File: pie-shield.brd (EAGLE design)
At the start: 35.1 x 25.2 mm, 21 parts, among them IC1 MAX481CSA, IC4 NRF24L01SMD, Q2 3.2X2.5CRYSTAL

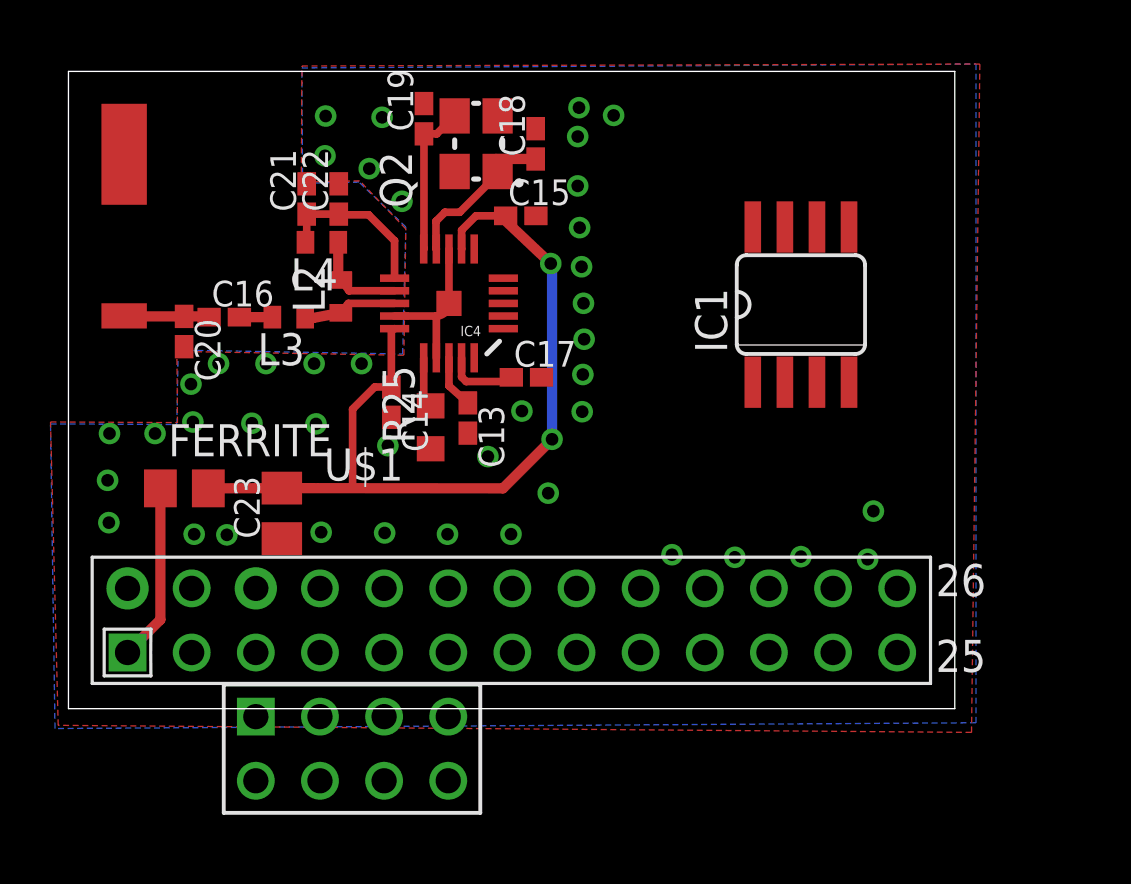
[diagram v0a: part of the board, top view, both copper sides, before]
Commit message: 1 square inch reached
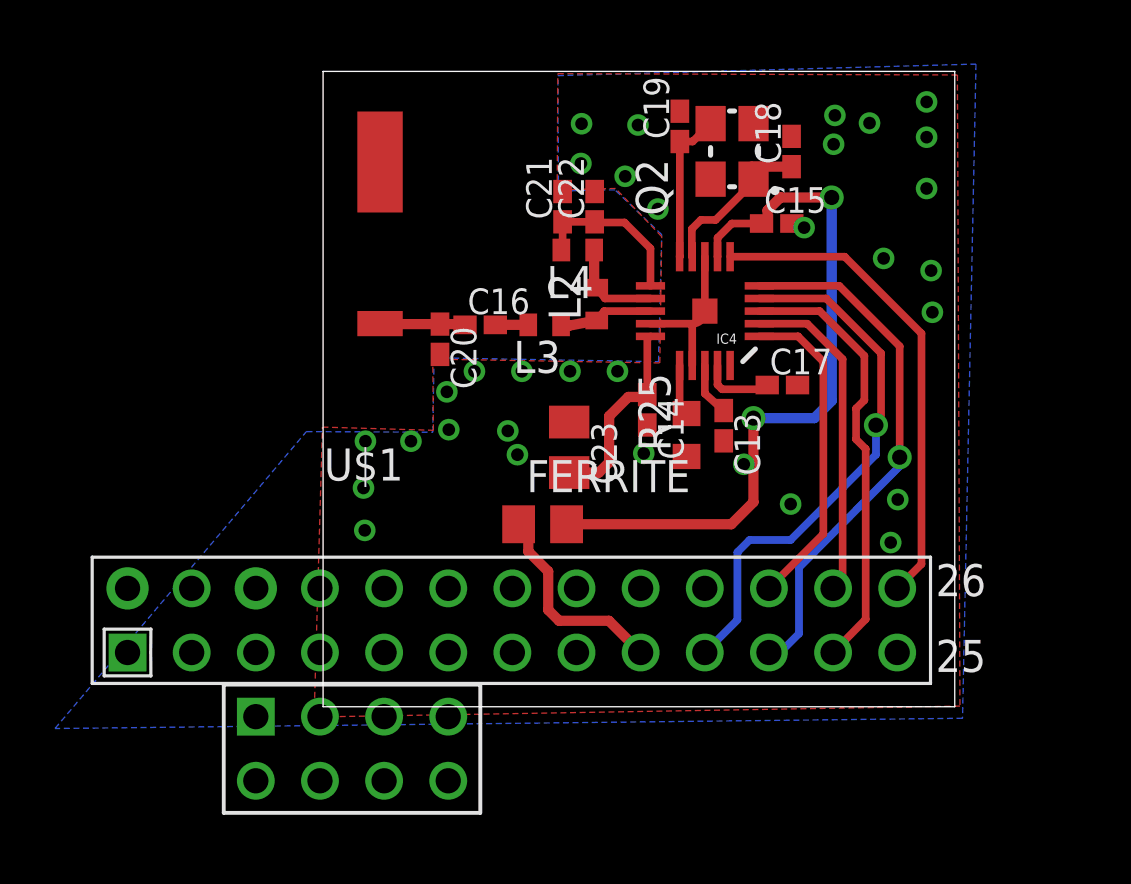
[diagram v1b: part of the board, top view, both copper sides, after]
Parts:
- removed IC1: MAX481CSA, maxim:SO08
- moved FERRITE 14.3 mm to (18.8, 8.98)
- moved C23 11.7 mm to (19.8, 12.0), turned to 270 degrees
- moved C15 10.1 mm to (28.0, 20.9)
- moved C17 10.1 mm to (28.3, 14.5)
- moved C21 10.1 mm to (19.6, 21.6)
- moved Q2 10.1 mm to (26.3, 23.7)
- moved C19 10.1 mm to (24.2, 24.7)
- moved C20 10.1 mm to (14.7, 16.3)
- moved C22 10.1 mm to (20.8, 21.6)
- moved IC4 10.1 mm to (25.2, 17.4)
- moved L2 10.1 mm to (20.9, 17.7)
- moved L3 10.1 mm to (18.9, 16.9)
- moved R25 10.1 mm to (24.5, 12.5)
- moved ANT 10.1 mm to (12.3, 19.4)
- moved C13 10.1 mm to (26.0, 12.9)
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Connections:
- removed net N$2: U$1.P1_26
- removed net N$5: U$1.P1_22
- removed net VCC: IC1.8
- net +3V3: now also U$1.P1_17; no longer U$1.P1_1
- net CE: now also U$1.P1_22
- net CSN: now also U$1.P1_24
- net GND: now also U$1.P1_25; no longer IC1.5
- net IRQ: now also U$1.P1_26
- net N$1: now also U$1.P1_15; no longer U$1.P1_25
- net N$3: now also U$1.P1_18; no longer U$1.P1_17
- net N$4: now also U$1.P1_16; no longer U$1.P1_24
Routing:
- net MOSI: track 0.00 -> 21.4 mm, vias 0 -> 1
- net MISO: track 0.00 -> 21.1 mm, vias 0 -> 1
- net IRQ: track 0.00 -> 19.3 mm
- net SCK: track 0.00 -> 17.5 mm
- net CSN: track 0.00 -> 13.1 mm
- net CE: track 0.00 -> 12.8 mm
- net +3V3: track 7.04 -> 8.24 mm
- net +3V3_RF: track 39.1 -> 38.6 mm
- net GND: vias 42 -> 32
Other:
- board size 35.1 x 25.2 mm -> 25 x 25.2 mm
